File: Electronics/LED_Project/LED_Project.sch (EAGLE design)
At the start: 15 parts, among them IC1 7805T

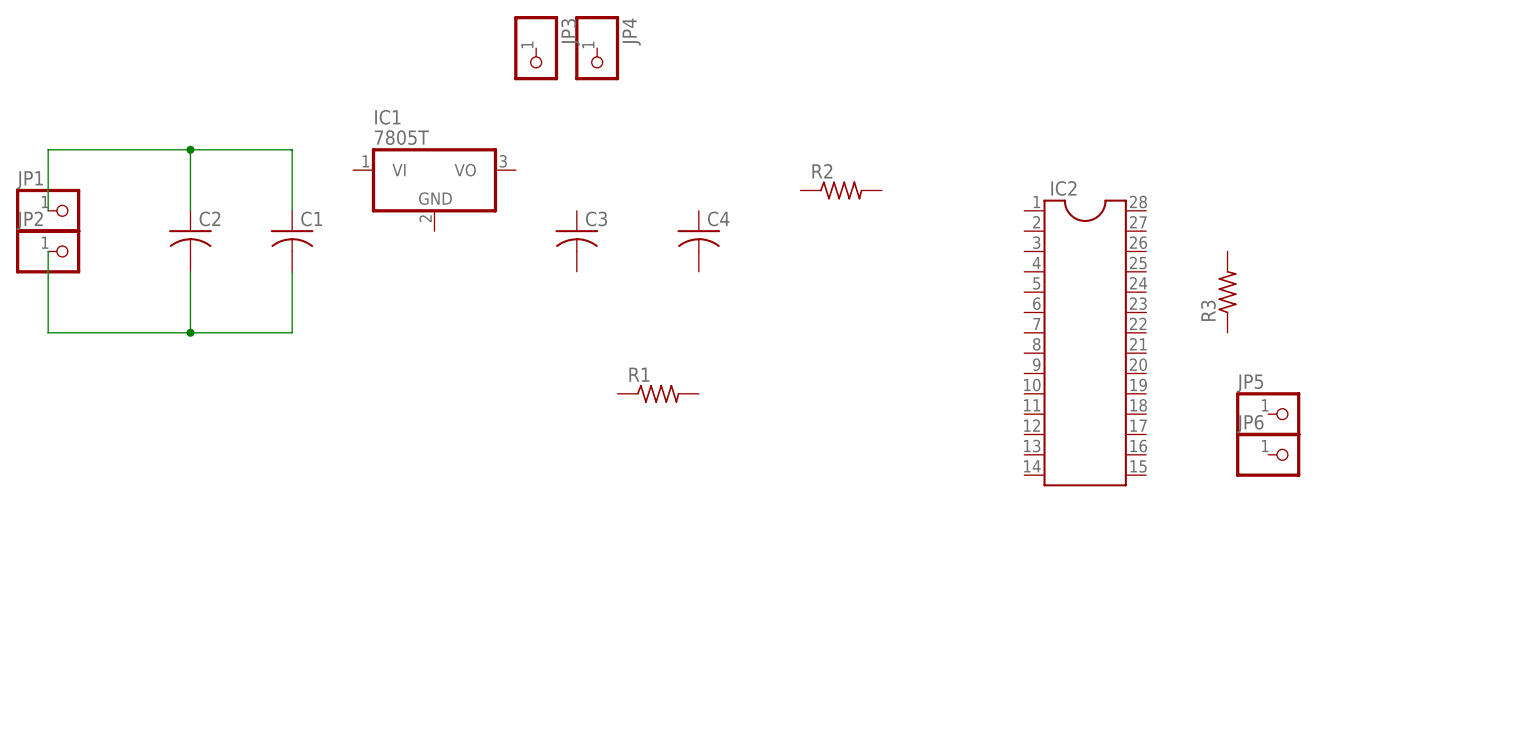
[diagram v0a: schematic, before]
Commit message: replacecd ECAD files
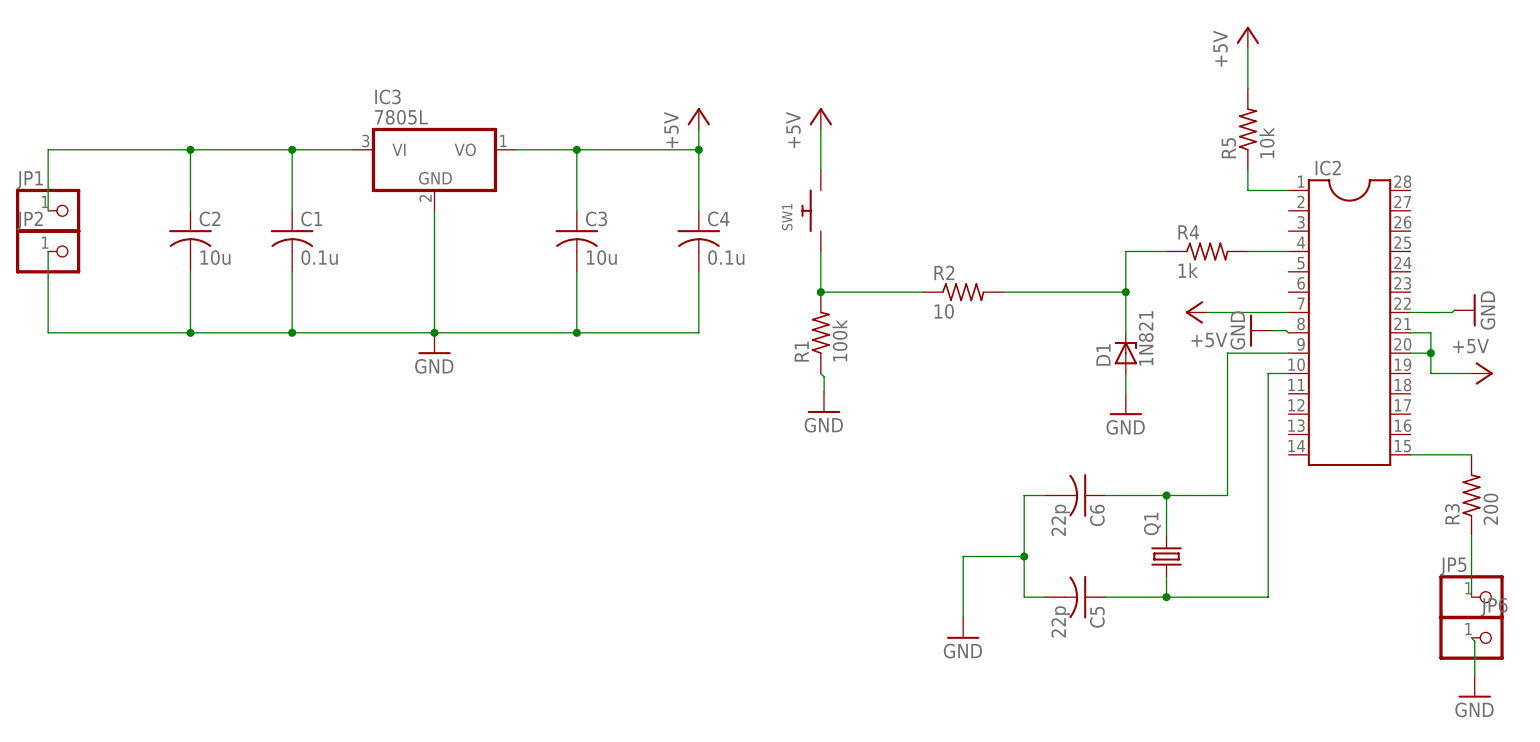
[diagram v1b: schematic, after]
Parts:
- removed IC1: 7805T, linear:7805T
- removed JP3, JP4: (no value), adafruit:PINHD-1X1
- added C5, C6: 22p, adafruit:C-USC0805K
- added D1: 1N821, diode:1N821
- added IC3: 7805L, adafruit:7805L
- added Q1: (no value), adafruit:CRYSTALHC49S
- added R4: 1k, adafruit:R-US_R0805
- added R5: 10k, adafruit:R-US_R0805
- added SW1: (no value), adafruit:SWITCH_PUSHBUTTONSOFTTOUCHSMD_SJ
- C1, C4: value (none) -> 0.1u
- C2, C3: value (none) -> 10u
- R1: value (none) -> 100k
- R2: value (none) -> 10
- R3: value (none) -> 200
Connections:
- new net +5V: C3.1, C4.1, IC2.20, IC2.21, IC2.7, IC3.VO, R5.2, SW1.P$2
- new net GND: C1.2, C2.2, C3.2, C4.2, C5.2, C6.2, D1.A, IC2.22, IC2.8, IC3.GND, JP2.1, JP6.1, R1.1
- new net N$10: C5.1, IC2.10, Q1.1
- new net N$12: IC2.1, R5.1
- new net N$2: R1.2, R2.1, SW1.P$1
- new net N$4: C6.1, IC2.9, Q1.2
- new net N$5: D1.C, R2.2, R4.1
- new net N$6: IC2.15, R3.2
- new net N$7: JP5.1, R3.1
- net N$1: now also IC3.VI
- net N$3: now also IC2.4, R4.2; no longer C1.2, C2.2, JP2.1
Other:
- moved on the sheet: IC2, JP5, JP6, R1, R2, R3
